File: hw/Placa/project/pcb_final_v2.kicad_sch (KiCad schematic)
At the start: 26 parts, among them J1 pin_socket-bluepill, J10 tcrt5000_conector_2, J11 tcrt5000_conector_3, J12 tcrt5000_conector_1, J2 pin_socket-bluepill, J9 tof-connector_3, SW2 key, U1 YAAJ_BluePill, U2 Receptor IR, U4 AMS1117-3.3

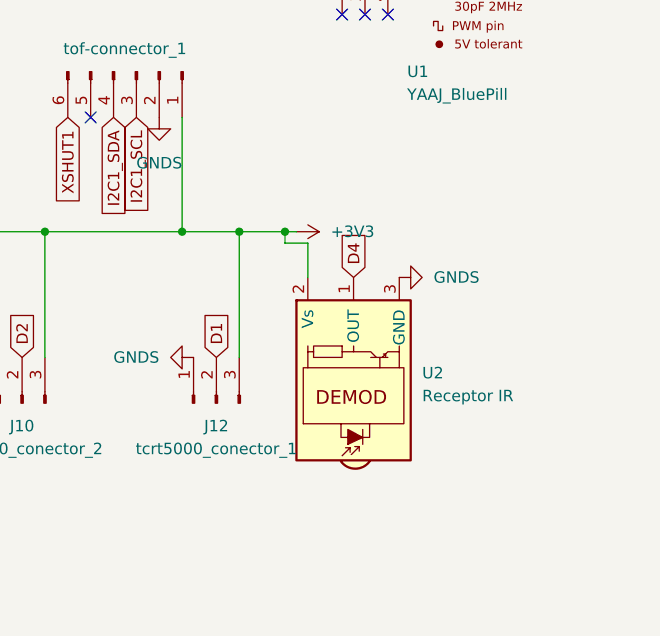
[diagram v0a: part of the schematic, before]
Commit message: pcb finalizada
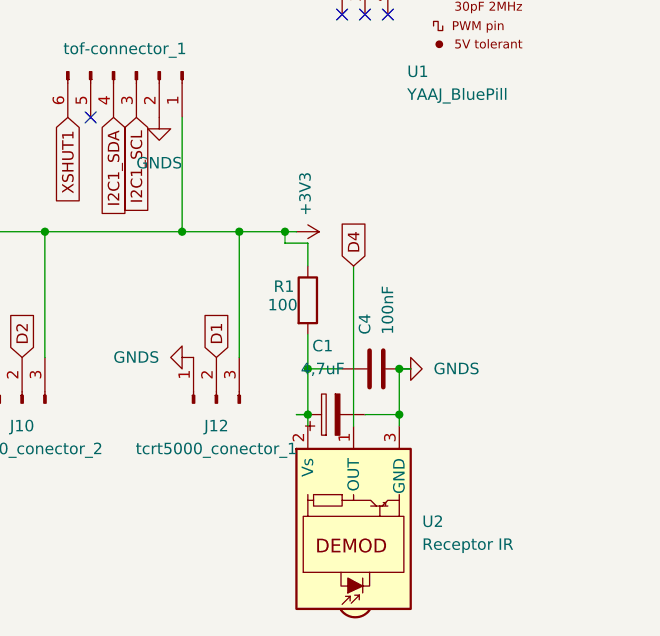
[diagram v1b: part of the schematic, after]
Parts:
- added C1: 4,7uF, Capacitor_SMD:C_0805_2012Metric_Pad1.18x1.45mm_HandSolder, symbol Device:C_Polarized
- added C4: 100nF, Capacitor_SMD:C_0805_2012Metric_Pad1.18x1.45mm_HandSolder, symbol Device:C
- added R1: 100, Resistor_SMD:R_0805_2012Metric, symbol Device:R
- C2, C3: footprint Capacitor_SMD:C_0805_2012Metric -> Capacitor_SMD:C_0805_2012Metric_Pad1.18x1.45mm_HandSolder
- SW2: footprint Button_Switch_THT:SW_DIP_SPSTx01_Slide_6.7x4.1mm_W7.62mm_P2.54mm_LowProfile -> Button_Switch_THT:SW_CK_JS202011CQN_DPDT_Straight
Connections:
- net +3V3: now also R1.1; no longer U2.2 (Vs)
- net GNDS: now also C1.2, C4.1
- new net: C1.1, C4.2, R1.2, U2.2 (Vs)
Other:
- moved on the sheet: U2
